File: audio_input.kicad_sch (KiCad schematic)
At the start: 14 parts, among them J5 extra_input, J6 AudioJack4

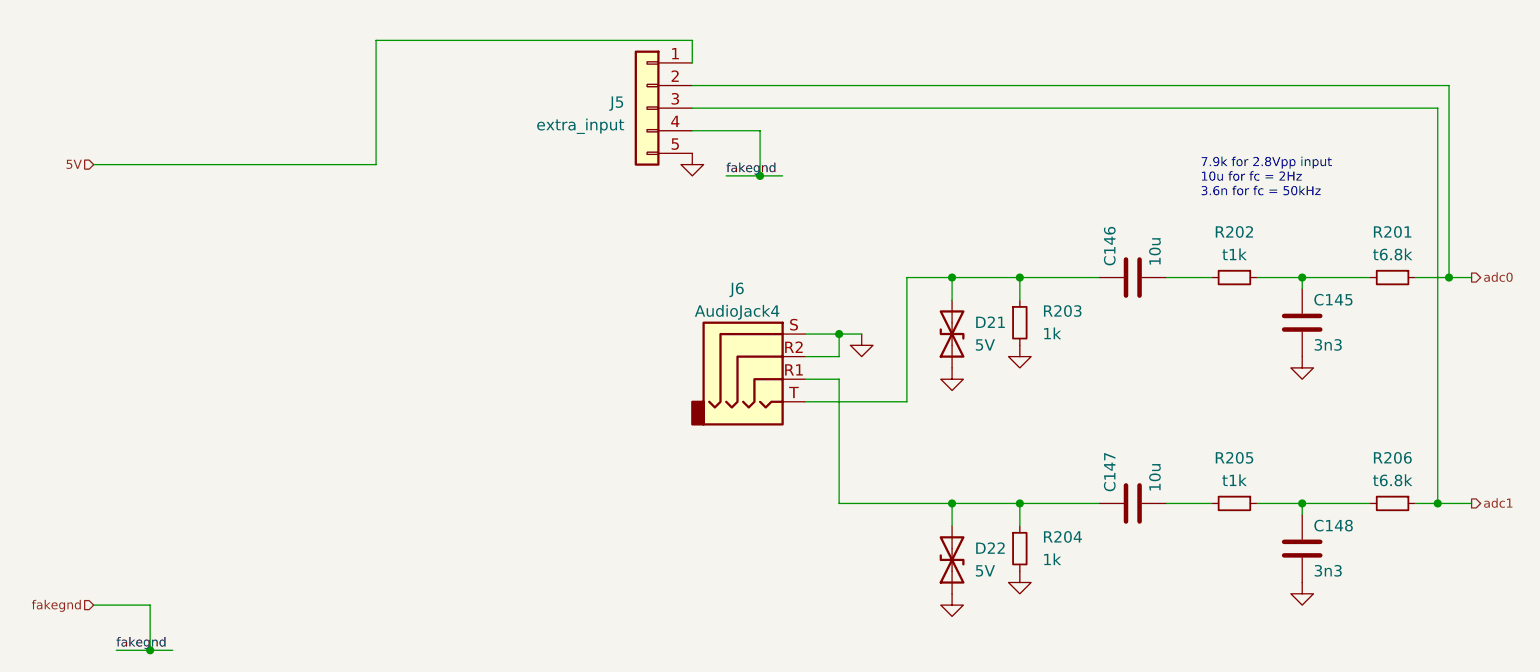
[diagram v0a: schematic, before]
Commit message: all known bugs fixed
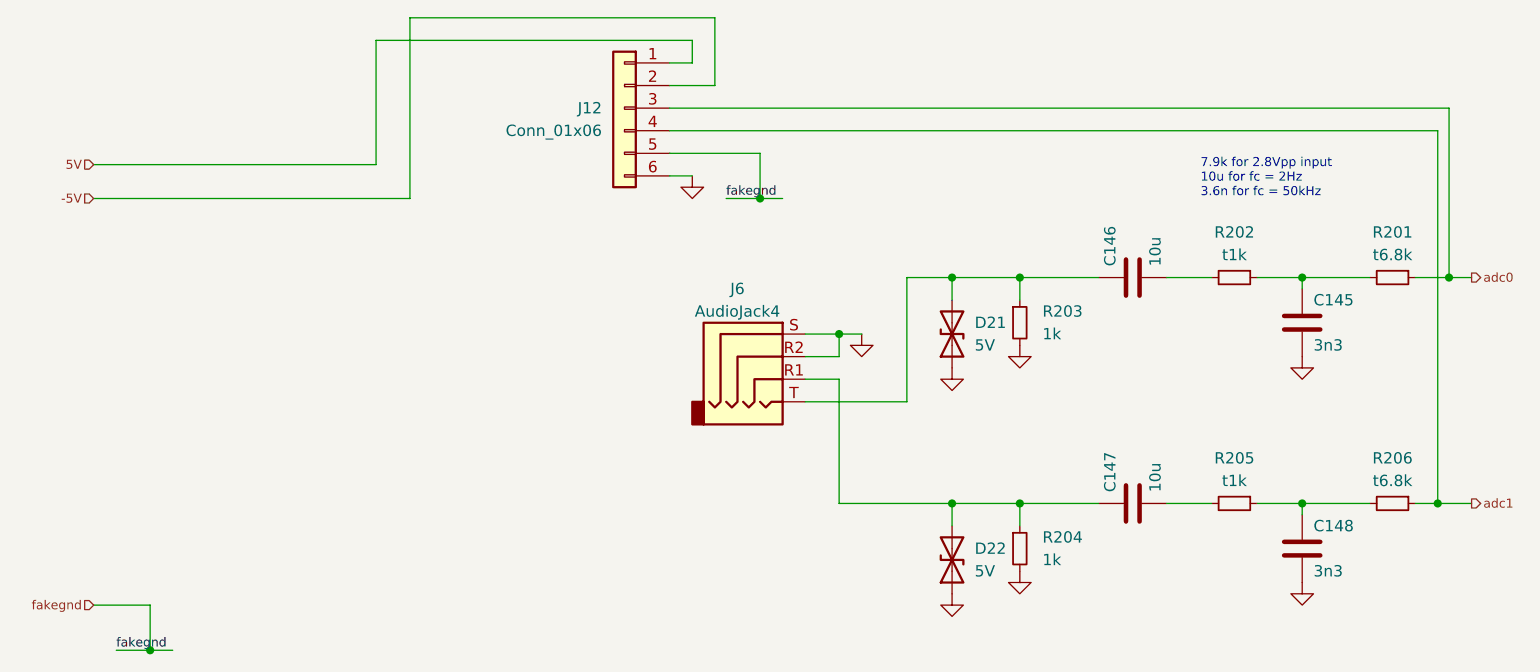
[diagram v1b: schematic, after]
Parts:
- removed J5: extra_input, Connector_JST:JST_GH_BM05B-GHS-TBT_1x05-1MP_P1.25mm_Vertical, symbol Connector_Generic:Conn_01x05
- added J12: Conn_01x06, Connector_JST:JST_GH_BM06B-GHS-TBT_1x06-1MP_P1.25mm_Vertical, symbol Connector_Generic:Conn_01x06
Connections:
- net 5V: now also J12.1 (Pin_1)
- net GND: now also J12.6 (Pin_6)
- net adc0: now also J12.3 (Pin_3)
- net adc1: now also J12.4 (Pin_4)
- net fakegnd: now also J12.5 (Pin_5)
- new net -5V: J12.2 (Pin_2)
